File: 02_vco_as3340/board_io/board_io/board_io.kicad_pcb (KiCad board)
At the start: 2 copper layers, 48.8 x 55 mm, 9 parts, among them J1 Conn_02x05_Odd_Even, J2 Conn_02x04_Odd_Even, SW2 SW_SPDT

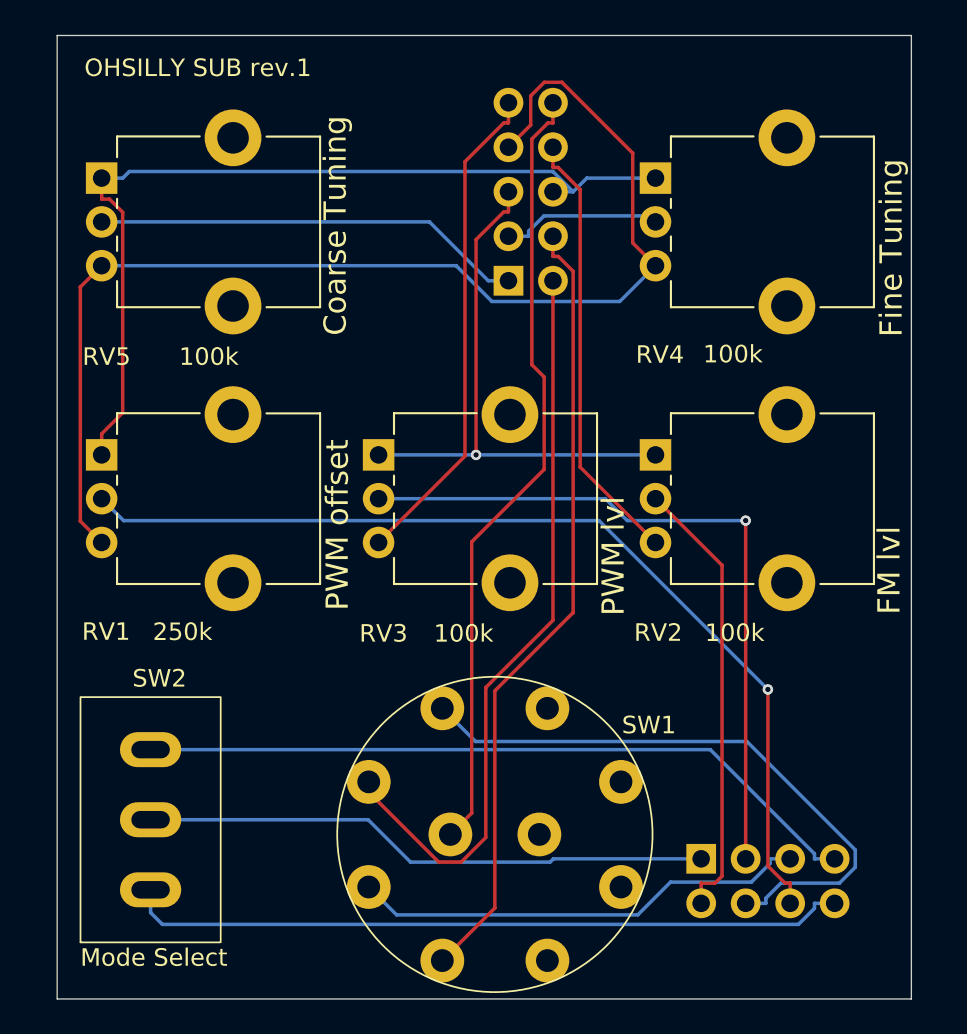
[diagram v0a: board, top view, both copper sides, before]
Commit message: final tweaks
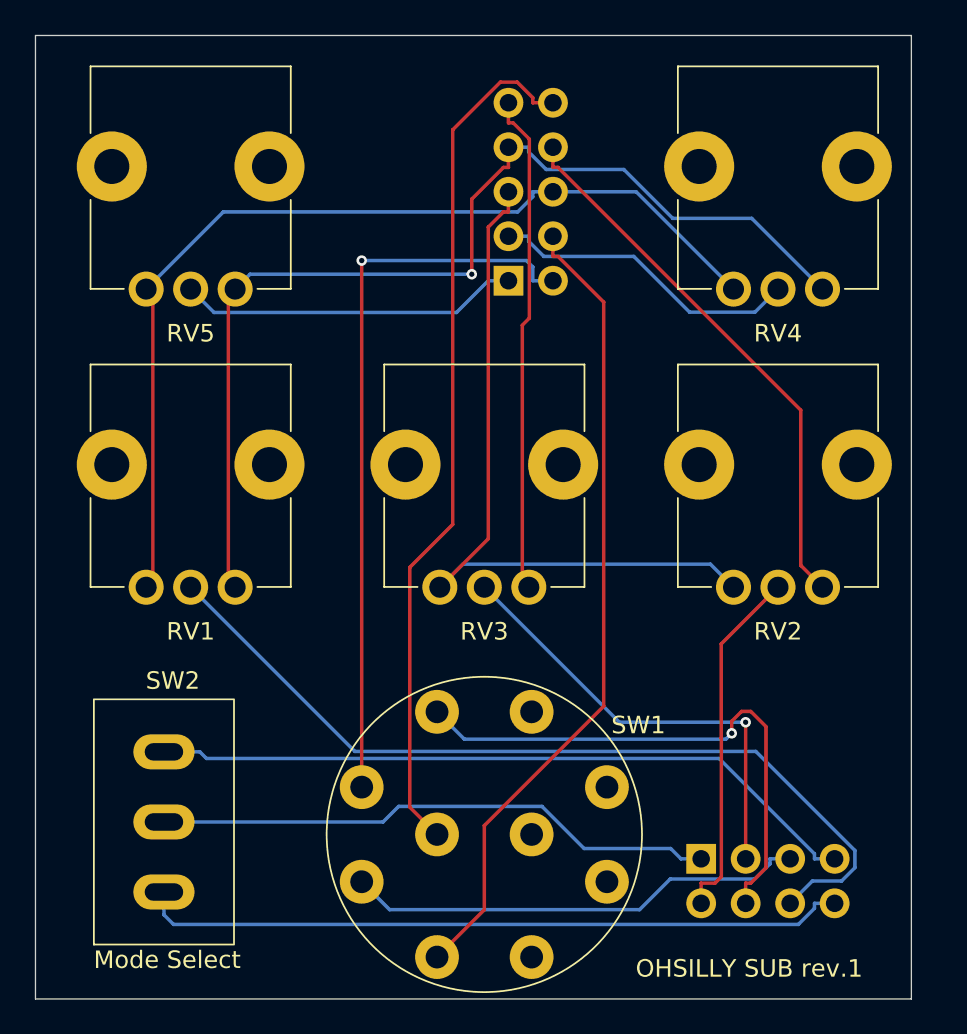
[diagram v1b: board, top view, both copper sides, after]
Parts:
- RV1, RV2, RV3, RV4, RV5: footprint Potentiometer_THT:Potentiometer_Alpha_RD901F-40-00D_Single_Vertical_CircularHoles -> cynthia:pot
- moved RV4 7.02 mm to (55.8, 25.8)
- moved RV2 7.01 mm to (55.8, 42.8)
- moved RV3 6.06 mm to (39.1, 42.8)
- moved RV5 5.12 mm to (22.3, 25.8)
- moved RV1 5.11 mm to (22.3, 42.8)
- moved SW2 0.77 mm to (20.8, 63.2)
- moved SW1 0.60 mm to (39.1, 63.9)
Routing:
- net PWM CV Levelled: track 40.8 -> 25.9 mm
- net GND: track 31.8 -> 42.2 mm, vias 1 -> 0
- net Fine Tuning: track 9.18 -> 17.9 mm
- net +12V: track 68.4 -> 60.9 mm, vias 0 -> 1
- net FM CV Hot: track 25.2 -> 31.7 mm
- net PWM Offset: track 55.4 -> 49.7 mm, vias 1 -> 0
- net FM CV Levelled: track 25.6 -> 20.3 mm
- net Coarse Tuning: track 24.6 -> 19.4 mm
- net -12V: track 50.8 -> 55.6 mm
- net Sync COM: track 44.9 -> 49.4 mm
- net Soft Sync: track 35.2 -> 31.6 mm, vias 0 -> 1
- net Hard Sync +: track 45.1 -> 46.5 mm
- net Hard Sync -: track 42.9 -> 41.9 mm, vias 0 -> 1
- net Mode VCO: track 41.8 -> 41.0 mm
- net Mode LFO: track 41.3 -> 40.5 mm
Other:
- board size 48.8 x 55 mm -> 50 x 55 mm
